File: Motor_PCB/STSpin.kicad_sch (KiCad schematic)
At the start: 1 part, among them U1 STSPIN32G4

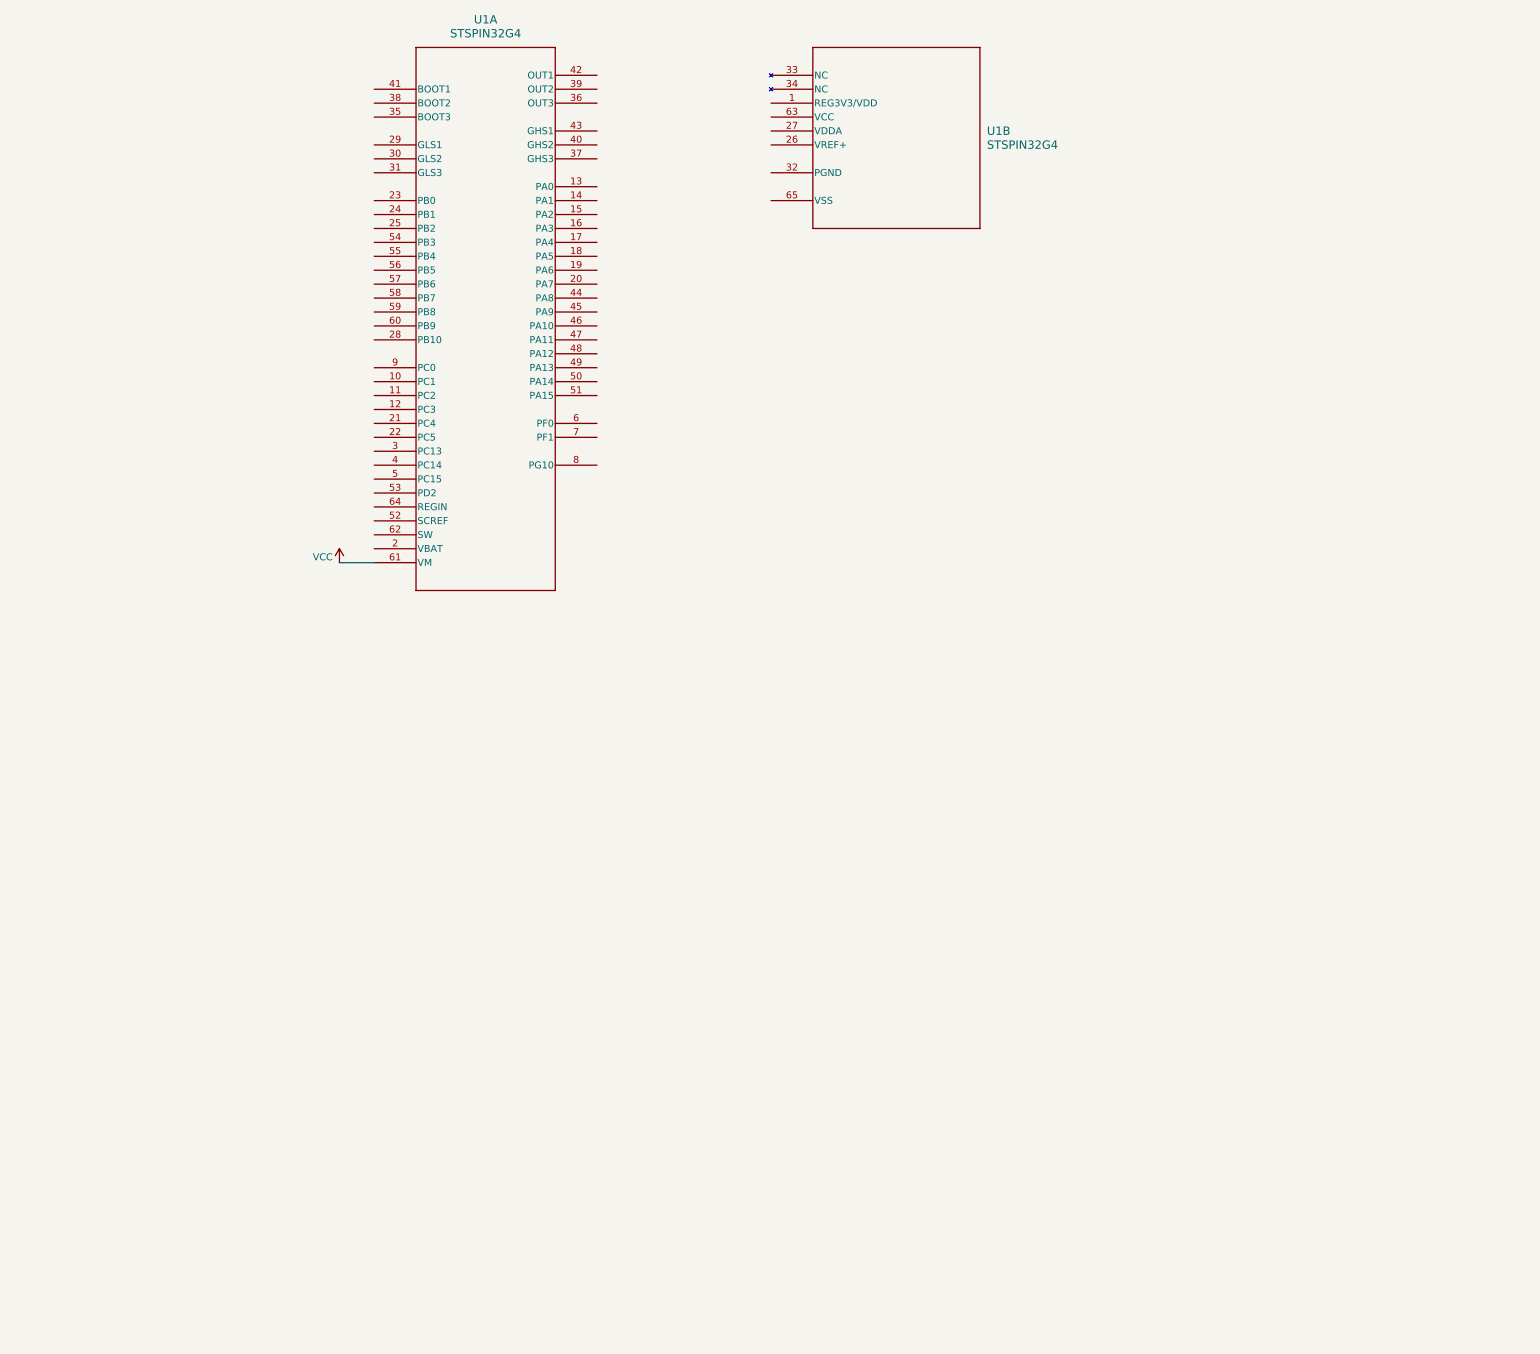
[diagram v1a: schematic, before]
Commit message: Schematics mostly done
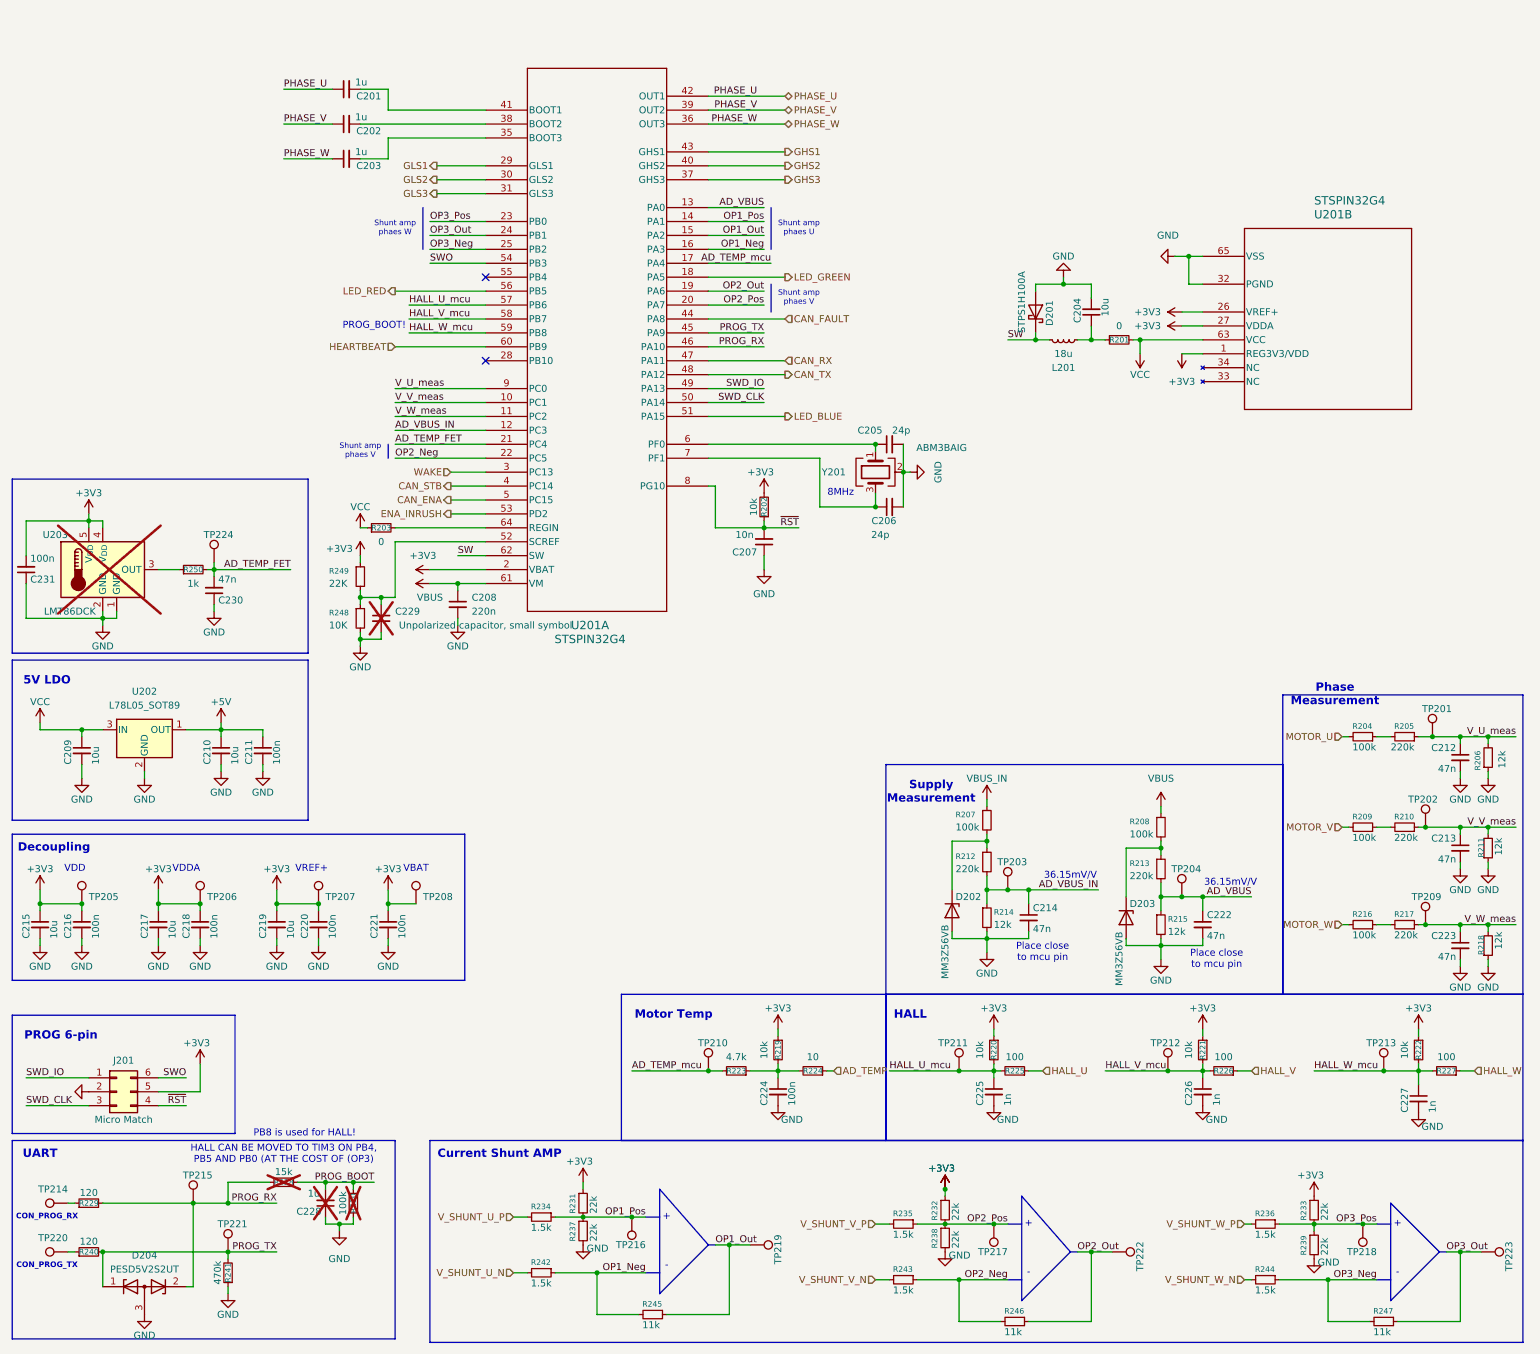
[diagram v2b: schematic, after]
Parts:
- added C201, C202, C203: 1u, symbol Device:C_Small
- added C204, C209, C210, C215, C217, C219: 10u, symbol Device:C_Small
- added C205, C206: 24p, Capacitor_SMD:C_0603_1608Metric, symbol Device:C_Small
- added C207: 10n, Capacitor_SMD:C_0603_1608Metric, symbol Device:C_Small
- added C208, C229: 220n, symbol Device:C_Small
- added C211, C216, C218, C220, C221, C224: 100n, symbol Device:C_Small
- added C212, C213, C214, C222, C223, C230: 47n, Capacitor_SMD:C_0603_1608Metric, symbol Device:C_Small
- added C225, C226, C227: 1n, symbol Device:C_Small
- added C228: 1u, Capacitor_SMD:C_0603_1608Metric, symbol Device:C_Small
- added C231: 100n, Capacitor_SMD:C_0603_1608Metric, symbol Device:C_Small
- added D201: STPS1H100A, symbol Device:D_Schottky
- added D202, D203: MM3Z56VB, Diode_SMD:D_SMA, symbol Diode:MM3Zxx
- added D204: PESD5V2S2UT, Package_TO_SOT_SMD:SOT-23, symbol Device:D_Zener_Dual_CommonAnode_KKA
- added J201: Micro Match, MOTOR_PCB:CONN6_7-188275-6_TEC, symbol Connector_Generic:Conn_02x03_Counter_Clockwise
- added L201: 18u, symbol Device:L_Small
- added R201, R203: 0, symbol Device:R_Small
- added R202: 10k, Resistor_SMD:R_0603_1608Metric, symbol Device:R_Small
- added R204, R207, R208, R209, R216, R230: 100k, Resistor_SMD:R_0603_1608Metric, symbol Device:R_Small
- added R205, R210, R212, R213, R217: 220k, Resistor_SMD:R_0603_1608Metric, symbol Device:R_Small
- added R206, R211, R214, R215, R218: 12k, Resistor_SMD:R_0603_1608Metric, symbol Device:R_Small
- added R219, R220, R221, R222: 10k, symbol Device:R_Small
- added R223: 4.7k, symbol Device:R_Small
- added R224: 10, symbol Device:R_Small
- added R225, R226, R227: 100, symbol Device:R_Small
- added R228: 15k, Resistor_SMD:R_0603_1608Metric, symbol Device:R_Small
- added R229, R240: 120, Resistor_SMD:R_0603_1608Metric, symbol Device:R_Small
- added R231, R232, R233, R237, R238, R239: 22k, Resistor_SMD:R_0603_1608Metric, symbol Device:R_Small
- added R234, R235, R236, R242, R243, R244: 1.5k, Resistor_SMD:R_0603_1608Metric, symbol Device:R_Small
- added R241: 470k, Resistor_SMD:R_0603_1608Metric, symbol Device:R_Small
- added R245, R246, R247: 11k, Resistor_SMD:R_0603_1608Metric, symbol Device:R_Small
- added R248: 10K, Resistor_SMD:R_0603_1608Metric, symbol Device:R_Small
- added R249: 22K, Resistor_SMD:R_0603_1608Metric, symbol Device:R_Small
- added R250: 1k, symbol Device:R_Small
- added TP201, TP202, TP203, TP204, TP205, TP206, TP207, TP208, TP209, TP210, TP211, TP212, TP213, TP214, TP215, TP216, TP217, TP218, TP219, TP220, TP221, TP222, TP223, TP224: TestPoint, TestPoint:TestPoint_Pad_D1.5mm, symbol Connector:TestPoint
- added U202: L78L05_SOT89, Package_TO_SOT_SMD:SOT-89-3, symbol Regulator_Linear:L78L05_SOT89
- added U203: LMT86DCK, Package_TO_SOT_SMD:SOT-353_SC-70-5, symbol Sensor_Temperature:LMT86DCK
- added Y201: ABM3BAIG, Crystal:Crystal_SMD_5032-4Pin_5.0x3.2mm, symbol Device:Crystal_GND24
- renumbered U1 to U201
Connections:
- net VCC: now also U201.63 (VCC), C209.1, R201.2, R203.1, U202.3 (IN); no longer U201.61 (VM)
- net +3V3: now reaches U201.1 (REG3V3/VDD)
- net +3V3: now also U201.2 (VBAT), U201.26 (VREF+), U201.27 (VDDA), C215.1, C216.1, C217.1, C218.1, C219.1, C220.1, C221.1, C231.2, J201.5 (Pin_5), R202.2, R219.1, R220.1, R221.1, R222.1, R231.1, R232.1, R233.1, R249.1, TP205.1, TP206.1, TP207.1, TP208.1, U203.4 (V_{DD}), U203.5 (V_{DD})
- net GND: now reaches U201.32 (PGND)
- net GND: now also U201.65 (VSS), C204.2, C205.2, C206.2, C207.1, C208.2, C209.2, C210.2, C211.2, C212.2, C213.2, C214.2, C215.2, C216.2, C217.2, C218.2, C219.2, C220.2, C221.2, C222.2, C223.2, C224.2, C225.2, C226.2, C227.2, C228.1, C229.2, C230.1, C231.1, D201.2 (A), D202.2 (A), D203.2 (A), D204.3 (A), J201.2 (Pin_2), R206.1, R211.1, R214.2, R215.2, R218.1, R230.1, R237.2, R238.2, R239.2, R241.1, R248.2, U202.2 (GND), U203.1 (GND), U203.2 (GND), Y201.2 (G), Y201.4 (G)
- net V_V_meas: now reaches U201.10 (PC1)
- net V_V_meas: now also C213.1, R210.1, R211.2, TP202.1
- net V_W_meas: now reaches U201.11 (PC2)
- net V_W_meas: now also C223.1, R217.1, R218.2, TP209.1
- net AD_VBUS_IN: now reaches U201.12 (PC3)
- net AD_VBUS_IN: now also C214.1, R212.2, R214.1, TP203.1
- net AD_VBUS: now reaches U201.13 (PA0)
- net AD_VBUS: now also C222.1, R213.2, R215.1, TP204.1
- net OP1_Pos: now reaches U201.14 (PA1)
- net OP1_Pos: now also R231.2, R234.1, R237.1, TP216.1
- net OP1_Out: now reaches U201.15 (PA2)
- net OP1_Out: now also R245.1, TP219.1
- net OP1_Neg: now reaches U201.16 (PA3)
- net OP1_Neg: now also R242.1, R245.2
- net AD_TEMP_mcu: now reaches U201.17 (PA4)
- net AD_TEMP_mcu: now also R223.2, TP210.1
- net LED_GREEN: now reaches U201.18 (PA5)
- net OP2_Out: now reaches U201.19 (PA6)
- net OP2_Out: now also R246.1, TP222.1
- net OP2_Pos: now reaches U201.20 (PA7)
- net OP2_Pos: now also R232.2, R235.1, R238.1, TP217.1
- net AD_TEMP_FET: now reaches U201.21 (PC4)
- net AD_TEMP_FET: now also C230.2, R250.2, TP224.1
- net OP2_Neg: now reaches U201.22 (PC5)
- net OP2_Neg: now also R243.1, R246.2
- net OP3_Pos: now reaches U201.23 (PB0)
- net OP3_Pos: now also R233.2, R236.1, R239.1, TP218.1
- net OP3_Out: now reaches U201.24 (PB1)
- net OP3_Out: now also R247.1, TP223.1
- net OP3_Neg: now reaches U201.25 (PB2)
- net OP3_Neg: now also R244.1, R247.2
- net GLS1: now reaches U201.29 (GLS1)
- net WAKE: now reaches U201.3 (PC13)
- net GLS2: now reaches U201.30 (GLS2)
- net GLS3: now reaches U201.31 (GLS3)
- net at U201.35 (BOOT3): now also C203.2
- net PHASE_W: now reaches U201.36 (OUT3)
- net PHASE_W: now also C203.1
- net GHS3: now reaches U201.37 (GHS3)
- net at U201.38 (BOOT2): now also C202.2
- net PHASE_V: now reaches U201.39 (OUT2)
- net PHASE_V: now also C202.1
- net CAN_STB: now reaches U201.4 (PC14)
- net GHS2: now reaches U201.40 (GHS2)
- net at U201.41 (BOOT1): now also C201.2
- net PHASE_U: now reaches U201.42 (OUT1)
- net PHASE_U: now also C201.1
- net GHS1: now reaches U201.43 (GHS1)
- net CAN_FAULT: now reaches U201.44 (PA8)
- net PROG_TX: now reaches U201.45 (PA9)
- net PROG_TX: now also D204.1 (K), R240.2, R241.2, TP221.1
- net PROG_RX: now reaches U201.46 (PA10)
- net PROG_RX: now also D204.2 (K), R228.1, R229.2, TP215.1
- net CAN_RX: now reaches U201.47 (PA11)
- net CAN_TX: now reaches U201.48 (PA12)
- net SWD_IO: now reaches U201.49 (PA13)
- net SWD_IO: now also J201.1 (Pin_1)
- net CAN_ENA: now reaches U201.5 (PC15)
- net SWD_CLK: now reaches U201.50 (PA14)
- net SWD_CLK: now also J201.3 (Pin_3)
- net LED_BLUE: now reaches U201.51 (PA15)
- net at U201.52 (SCREF): now also C229.1, R248.1, R249.2
- net ENA_INRUSH: now reaches U201.53 (PD2)
- net SWO: now reaches U201.54 (PB3)
- net SWO: now also J201.6 (Pin_6)
- net LED_RED: now reaches U201.56 (PB5)
- net HALL_U_mcu: now reaches U201.57 (PB6)
- net HALL_U_mcu: now also C225.1, R220.2, R225.2, TP211.1
- net HALL_V_mcu: now reaches U201.58 (PB7)
- net HALL_V_mcu: now also C226.1, R221.2, R226.2, TP212.1
- net HALL_W_mcu: now reaches U201.59 (PB8)
- net HALL_W_mcu: now also C227.1, R222.2, R227.2, TP213.1
- net at U201.6 (PF0): now also C205.1, Y201.1
- net HEARTBEAT: now reaches U201.60 (PB9)
- net SW: now reaches U201.62 (SW)
- net SW: now also D201.1 (K), L201.1
- net at U201.64 (REGIN): now also R203.2
- net at U201.7 (PF1): now also C206.1, Y201.3
- net ~{RST}: now reaches U201.8 (PG10)
- net ~{RST}: now also C207.2, J201.4 (Pin_4), R202.1
- net V_U_meas: now reaches U201.9 (PC0)
- net V_U_meas: now also C212.1, R205.1, R206.2, TP201.1
- new net: C224.1, R219.2, R223.1, R224.2
- new net: C204.1, L201.2, R201.1
- new net: R204.1, R205.2
- new net: R229.1, TP214.1
- new net: D203.1 (K), R208.2, R213.1
- new net: R216.1, R217.2
- new net: R240.1, TP220.1
- new net: D202.1 (K), R207.2, R212.1
- new net: R250.1, U203.3 (OUT)
- new net: R209.1, R210.2
- new net +5V: C210.1, C211.1, U202.1 (OUT)
- new net AD_TEMP: R224.1
- new net HALL_U: R225.1
- new net HALL_V: R226.1
- new net HALL_W: R227.1
- new net MOTOR_U: R204.2
- new net MOTOR_V: R209.2
- new net MOTOR_W: R216.2
- new net PROG_BOOT: C228.2, R228.2, R230.2
- new net VBUS: C208.1, R208.1, U201.61 (VM)
- new net VBUS_IN: R207.1
- new net V_SHUNT_U_N: R242.2
- new net V_SHUNT_U_P: R234.2
- new net V_SHUNT_V_N: R243.2
- new net V_SHUNT_V_P: R235.2
- new net V_SHUNT_W_N: R244.2
- new net V_SHUNT_W_P: R236.2
- no-connect marks 0 -> 2
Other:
- note added: "+"
- note added: "-"
- note added: "36.15mV/V"
- note added: "5V LDO"
- note added: "8MHz"
- note added: "CON_PROG_RX"
- note added: "CON_PROG_TX"
- note added: "Current Shunt AMP"
- note added: "Decoupling"
- note added: "HALL"
- note added: "HALL CAN BE MOVED TO TIM3 ON PB4, PB5 AND PB0 (AT THE COST OF (OP3)"
- note added: "Motor Temp"
- note added: "PB8 is used for HALL!"
- note added: "PROG 6-pin"
- note added: "PROG_BOOT!"
- note added: "Phase Measurement"
- note added: "Place close to mcu pin"
- note added: "Shunt amp phaes U"
- note added: "Shunt amp phaes V"
- note added: "Shunt amp phaes W"
- note added: "Supply Measurement"
- note added: "UART"
- note added: "VBAT"
- note added: "VDD"
- note added: "VDDA"
- note added: "VREF+"
- moved on the sheet: U201A, U201B
